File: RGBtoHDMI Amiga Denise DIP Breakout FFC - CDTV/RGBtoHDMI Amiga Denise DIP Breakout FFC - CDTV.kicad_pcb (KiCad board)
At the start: 2 copper layers, 89.4 x 22.1 mm, 5 parts

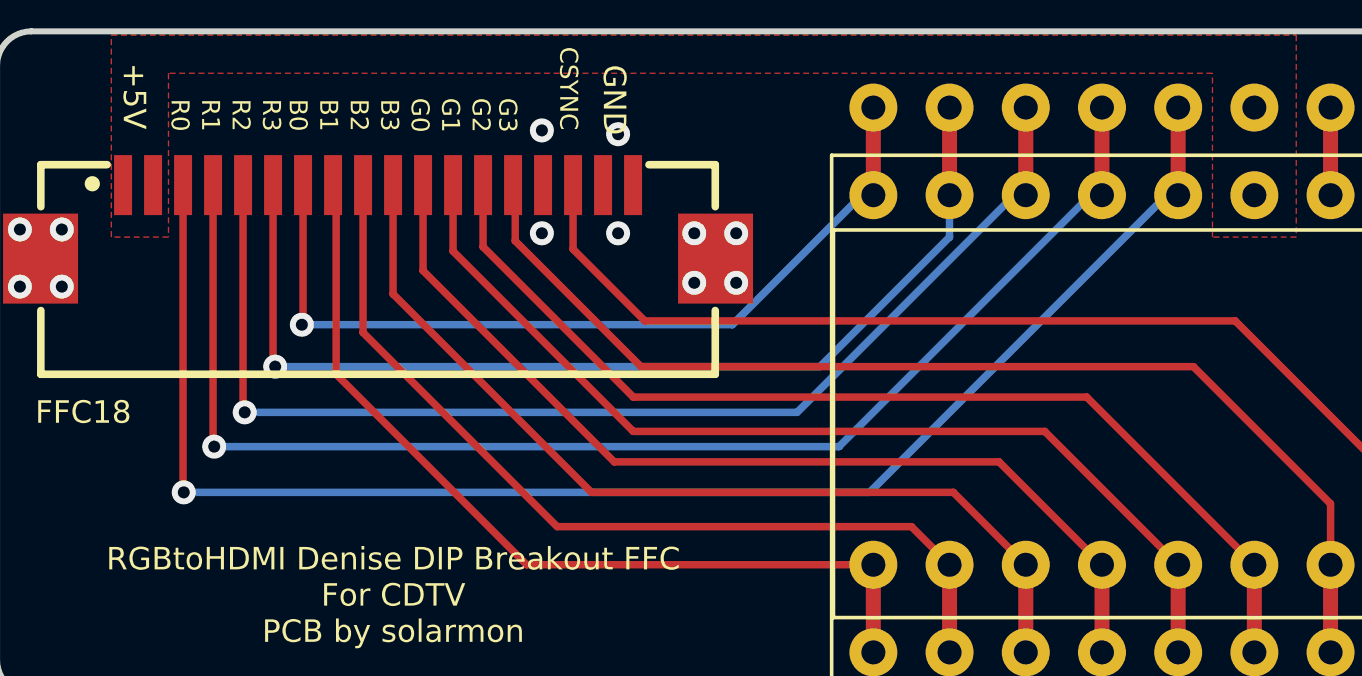
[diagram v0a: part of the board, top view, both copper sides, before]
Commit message: Tweaks
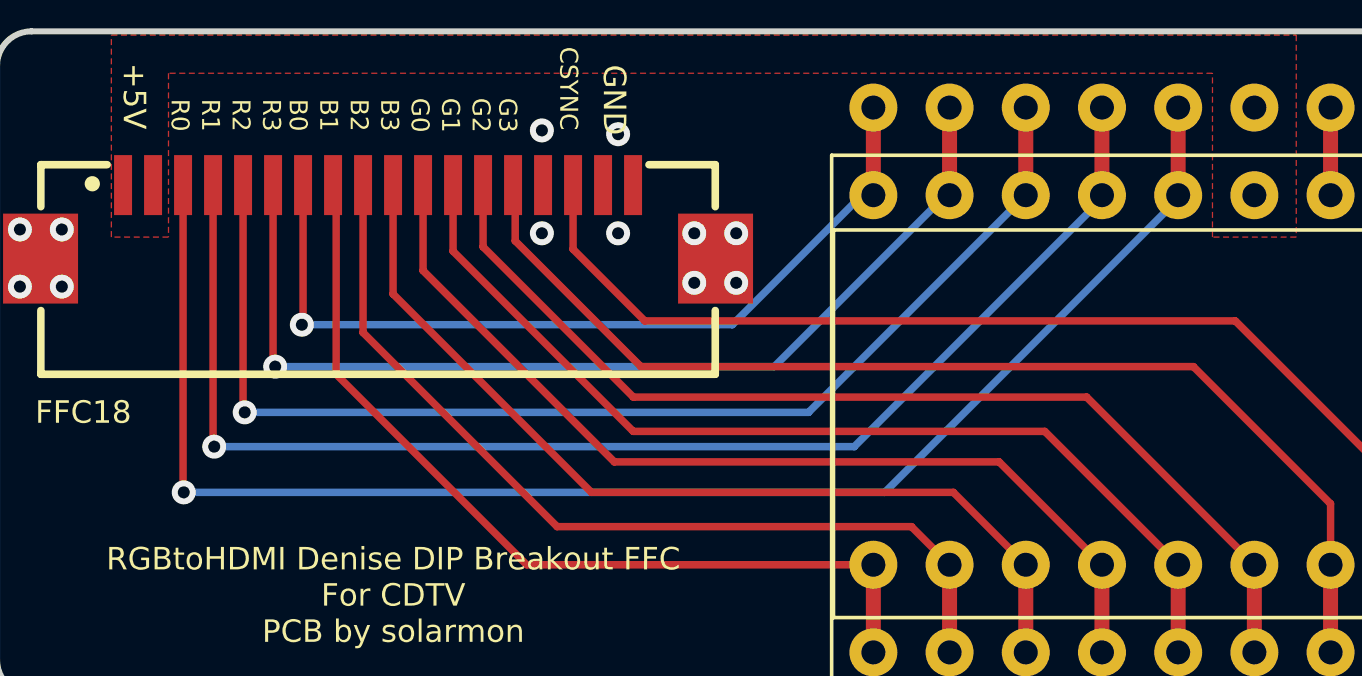
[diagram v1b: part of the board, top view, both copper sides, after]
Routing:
- net /R3: track 35.0 -> 34.2 mm
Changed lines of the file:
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@@
     (thickness 1.6)
     (drawings 25)
-    (tracks 120)
+    (tracks 125)
     (zones 0)
     (modules 5)
@@
   (title_block
     (title "RGBtoHDMI Denise Adapter - CDTV")
-    (date 2021-10-22)
+    (date 2021-11-18)
     (rev CDTV)
   )
@@
       (effects (font (size 1 1) (thickness 0.15)))
     )
-    (fp_text user %R (at 7.62 13.97 90) (layer F.Fab)
-      (effects (font (size 1 1) (thickness 0.15)))
-    )
-    (fp_arc (start 7.62 -1.33) (end 6.62 -1.33) (angle -180) (layer F.SilkS) (width 0.12))
     (fp_line (start 1.255 -1.27) (end 14.985 -1.27) (layer F.Fab) (width 0.1))
     (fp_line (start 14.985 -1.27) (end 14.985 29.21) (layer F.Fab) (width 0.1))
@@
     (fp_line (start 16.8 29.55) (end 16.8 -1.6) (layer F.CrtYd) (width 0.05))
     (fp_line (start 16.8 -1.6) (end -1.55 -1.6) (layer F.CrtYd) (width 0.05))
+    (fp_text user %R (at 7.62 13.97 90) (layer F.Fab)
+      (effects (font (size 1 1) (thickness 0.15)))
+    )
+    (fp_arc (start 7.62 -1.33) (end 6.62 -1.33) (angle -180) (layer F.SilkS) (width 0.12))
     (pad 24 thru_hole oval (at 15.24 0 270) (size 1.6 1.6) (drill 0.8) (layers *.Cu *.Mask)
       (net 39 "Net-(JDenise1-Pad24)"))
@@
   (segment (start 84.495 77.684) (end 84.455 77.724) (width 0.25) (layer F.Cu) (net 2))
   (segment (start 84.495 73.07) (end 84.495 77.684) (width 0.25) (layer F.Cu) (net 2))
+  (via (at 84.455 77.724) (size 0.8) (drill 0.4) (layers F.Cu B.Cu) (net 2))
   (segment (start 98.806 77.724) (end 84.455 77.724) (width 0.25) (layer B.Cu) (net 2))
-  (segment (start 103.505 73.025) (end 98.806 77.724) (width 0.25) (layer B.Cu) (net 2))
-  (via (at 84.455 77.724) (size 0.8) (drill 0.4) (layers F.Cu B.Cu) (net 2))
+  (segment (start 103.124 73.406) (end 98.806 77.724) (width 0.25) (layer B.Cu) (net 2))
+  (segment (start 103.505 73.406) (end 103.124 73.406) (width 0.25) (layer B.Cu) (net 2))
   (segment (start 106.045 70.485) (end 106.045 73.406) (width 0.5) (layer F.Cu) (net 3))
   (via (at 83.566 79.121) (size 0.8) (drill 0.4) (layers F.Cu B.Cu) (net 3))
-  (segment (start 106.045 74.803) (end 101.727 79.121) (width 0.25) (layer B.Cu) (net 3))
-  (segment (start 101.727 79.121) (end 83.566 79.121) (width 0.25) (layer B.Cu) (net 3))
-  (segment (start 106.045 73.025) (end 106.045 74.803) (width 0.25) (layer B.Cu) (net 3))
   (segment (start 83.495 73.07) (end 83.495 79.05) (width 0.25) (layer F.Cu) (net 3))
   (segment (start 83.495 79.05) (end 83.566 79.121) (width 0.25) (layer F.Cu) (net 3))
+  (segment (start 106.045 73.025) (end 106.045 73.406) (width 0.25) (layer B.Cu) (net 3))
+  (segment (start 100.203 79.121) (end 83.566 79.121) (width 0.25) (layer B.Cu) (net 3))
+  (segment (start 105.918 73.406) (end 100.203 79.121) (width 0.25) (layer B.Cu) (net 3))
+  (segment (start 106.045 73.406) (end 105.918 73.406) (width 0.25) (layer B.Cu) (net 3))
   (segment (start 108.585 70.485) (end 108.585 73.406) (width 0.5) (layer F.Cu) (net 4))
   (via (at 82.550004 80.645) (size 0.8) (drill 0.4) (layers F.Cu B.Cu) (net 4))
-  (segment (start 108.585 73.025) (end 100.965 80.645) (width 0.25) (layer B.Cu) (net 4))
-  (segment (start 100.965 80.645) (end 82.550004 80.645) (width 0.25) (layer B.Cu) (net 4))
   (segment (start 82.495 73.07) (end 82.495 80.589996) (width 0.25) (layer F.Cu) (net 4))
   (segment (start 82.495 80.589996) (end 82.550004 80.645) (width 0.25) (layer F.Cu) (net 4))
+  (segment (start 101.346 80.645) (end 82.550004 80.645) (width 0.25) (layer B.Cu) (net 4))
+  (segment (start 108.585 73.406) (end 101.346 80.645) (width 0.25) (layer B.Cu) (net 4))
+  (segment (start 108.585 73.025) (end 108.585 73.406) (width 0.25) (layer B.Cu) (net 4))
   (segment (start 111.125 70.485) (end 111.125 73.406) (width 0.5) (layer F.Cu) (net 5))
   (segment (start 81.495 81.749) (end 81.534 81.788) (width 0.25) (layer F.Cu) (net 5))
   (segment (start 81.495 73.07) (end 81.495 81.749) (width 0.25) (layer F.Cu) (net 5))
-  (segment (start 102.362 81.788) (end 81.534 81.788) (width 0.25) (layer B.Cu) (net 5))
-  (segment (start 111.125 73.025) (end 102.362 81.788) (width 0.25) (layer B.Cu) (net 5))
   (via (at 81.534 81.788) (size 0.8) (drill 0.4) (layers F.Cu B.Cu) (net 5))
+  (segment (start 102.87 81.788) (end 81.534 81.788) (width 0.25) (layer B.Cu) (net 5))
+  (segment (start 111.125 73.533) (end 102.87 81.788) (width 0.25) (layer B.Cu) (net 5))
+  (segment (start 111.125 73.406) (end 111.125 73.533) (width 0.25) (layer B.Cu) (net 5))
   (segment (start 113.665 70.485) (end 113.665 73.406) (width 0.5) (layer F.Cu) (net 6))
   (via (at 80.518006 83.312) (size 0.8) (drill 0.4) (layers F.Cu B.Cu) (net 6))
-  (segment (start 103.378 83.312) (end 80.518006 83.312) (width 0.25) (layer B.Cu) (net 6))
-  (segment (start 113.665 73.025) (end 103.378 83.312) (width 0.25) (layer B.Cu) (net 6))
   (segment (start 80.495 73.07) (end 80.495 83.288994) (width 0.25) (layer F.Cu) (net 6))
   (segment (start 80.495 83.288994) (end 80.518006 83.312) (width 0.25) (layer F.Cu) (net 6))
+  (segment (start 103.886 83.312) (end 80.518006 83.312) (width 0.25) (layer B.Cu) (net 6))
+  (segment (start 113.665 73.533) (end 103.886 83.312) (width 0.25) (layer B.Cu) (net 6))
+  (segment (start 113.665 73.025) (end 113.665 73.533) (width 0.25) (layer B.Cu) (net 6))
   (segment (start 146.685 85.725) (end 146.685 88.646) (width 0.5) (layer F.Cu) (net 8))
   (segment (start 144.145 85.725) (end 144.145 88.646) (width 0.5) (layer F.Cu) (net 9))
